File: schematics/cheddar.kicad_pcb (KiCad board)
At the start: 2 copper layers, 43 x 26 mm, 30 parts, among them J1 USB_OTG, J2 Conn_01x08, J3 Conn_01x08, J4 EXTERNAL_TRIGGER, J5 BATT_CONN, Q1 MOSFET_PCH, SW1 SW_Push, U1 CH340G, U2 MCP73831, U3 ESP-12E, U4 HT7333, Y1 12Mhz

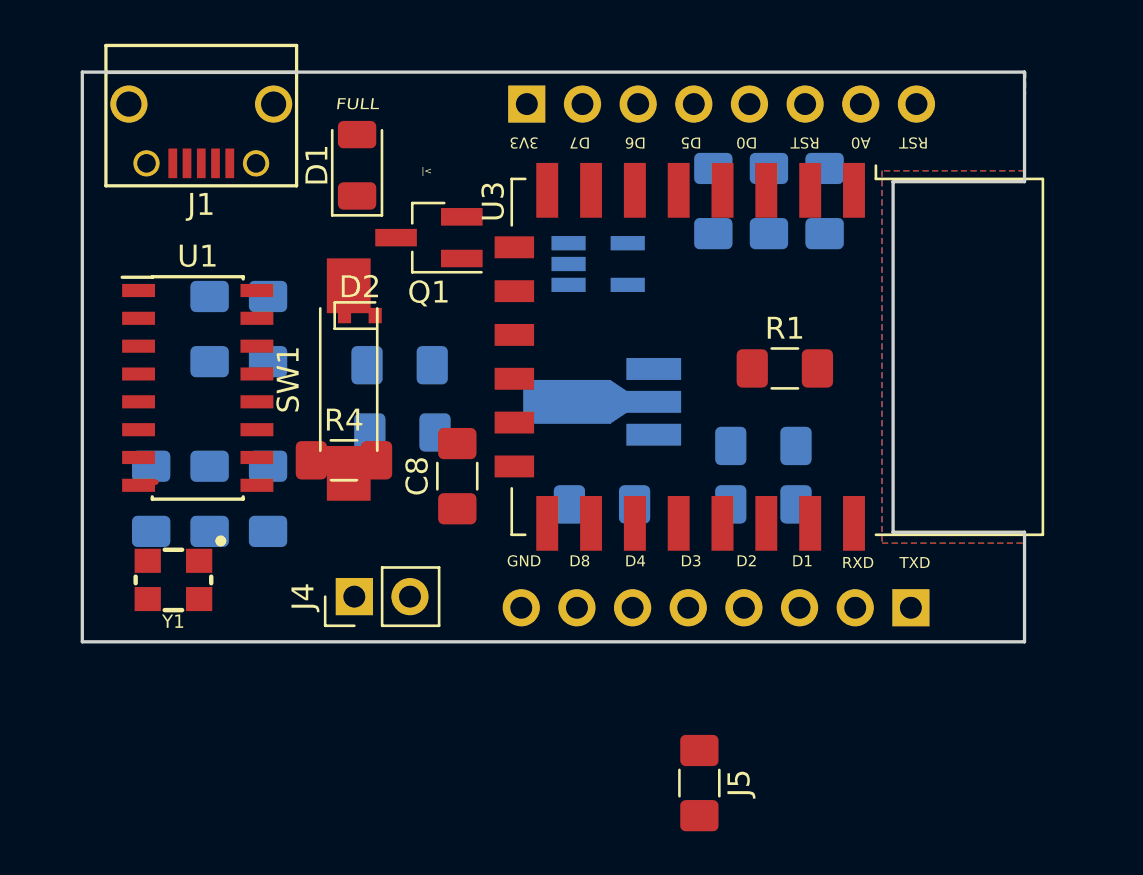
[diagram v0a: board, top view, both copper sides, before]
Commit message: Reestructure board
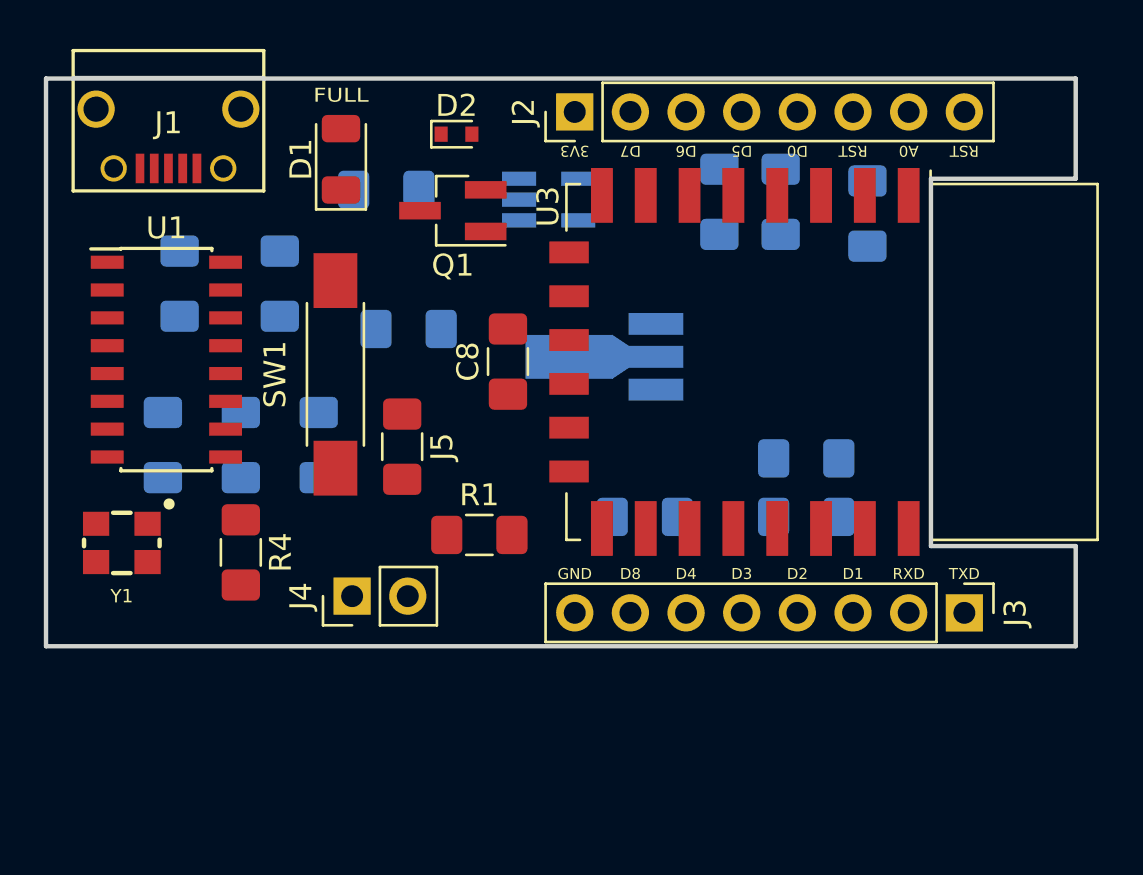
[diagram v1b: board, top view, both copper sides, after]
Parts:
- J2, J3: moved to F.Cu
- moved J5 20.5 mm to (147.0, 107.5)
- moved R1 15.9 mm to (150.5, 111.5)
- moved D2 9.38 mm to (149.4, 93.2)
- moved R2 8.03 mm to (146.2, 95.7)
- moved R4 6.31 mm to (139.6, 112.3), turned to 270 degrees
- moved C8 5.72 mm to (151.8, 103.6)
- moved R6 4.73 mm to (147.3, 102.1)
- moved U2 3.71 mm to (153.7, 96.2)
- moved C5 3.37 mm to (143.2, 107.4), turned to 270 degrees
- moved Y1 2.90 mm to (134.2, 111.8)
- moved C2 2.84 mm to (139.6, 107.4)
- moved C3 2.51 mm to (136.0, 107.4)
- moved U3 2.51 mm to (166.6, 103.6)
- moved C6 2.48 mm to (136.8, 100.0)
- moved J3 2.45 mm to (172.6, 115.0), turned to 270 degrees
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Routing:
- removed copper zone on F.Cu, net +5V
- removed copper zone on B.Cu, net GND
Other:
- board size 43 x 26 mm -> 47 x 25.9 mm
- board text removed: "|<"
